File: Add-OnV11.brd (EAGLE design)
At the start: 33.2 x 17.6 mm, 9 parts

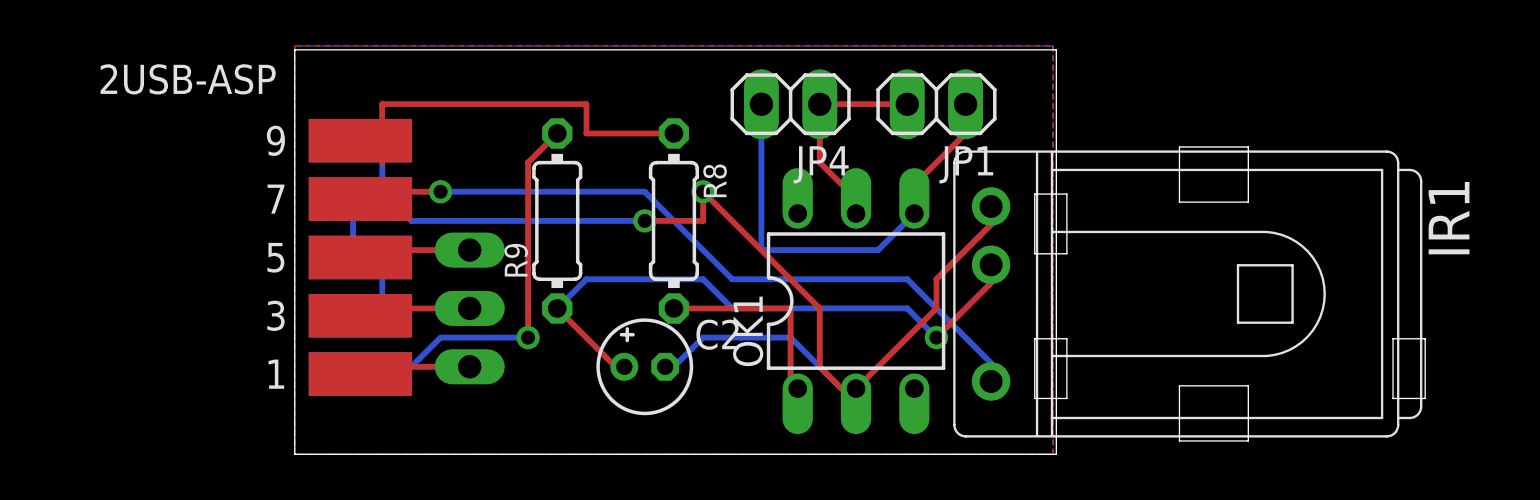
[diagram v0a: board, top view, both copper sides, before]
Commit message: Optimized
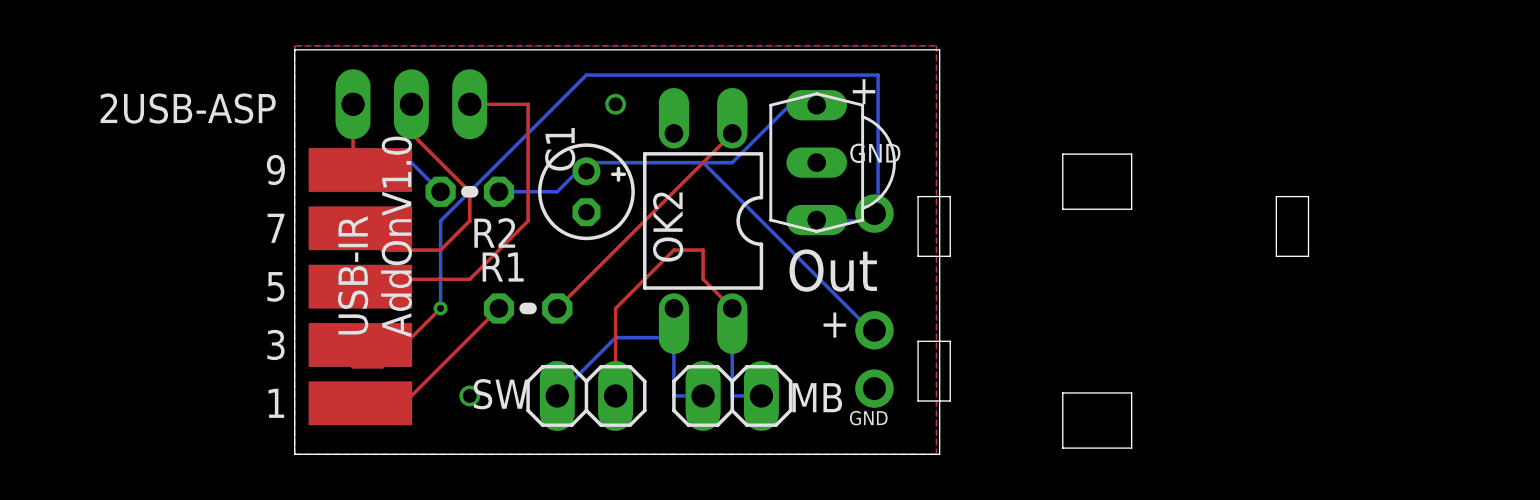
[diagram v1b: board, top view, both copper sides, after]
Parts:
- removed C2: 4,7uF, rcl:E1,8-4
- removed JP1, JP4: (no value), pinhead:1X02
- removed OK1: CNY17, optocoupler:DIL06
- removed R8: 100, rcl:0204/7
- removed R9: 560, rcl:0204/7
- added C1: 4,7uF, rcl:E1,8-4
- added MB, SW: (no value), pinhead:1X02
- added OK2: PC817, optocoupler:DIL04
- added R1: 100, rcl:0204V
- added R2: 560, rcl:0204V
- added U$1: TSOP1838, tsop-1:TSOP18XX
- moved FREI 9.25 mm to (5.08, 15.2), turned to 180 degrees
- moved IR1 5.09 mm to (25.2, 6.67), flipped to the bottom, turned to 0 degrees
- moved 2USB-ASP 1.27 mm to (2.86, 7.30)
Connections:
- removed net N$5: 2USB-ASP.P$2, R9.2
- removed net N$6: 2USB-ASP.P$5, FREI.1
- removed net N$7: 2USB-ASP.P$3, FREI.2
- removed net N$8: 2USB-ASP.P$1, FREI.3
- new net MOSI: 2USB-ASP.P$9, FREI.1
- new net NC: 2USB-ASP.P$7, FREI.2
- new net RST: 2USB-ASP.P$5, FREI.3
- new net VCC: 2USB-ASP.P$10, R2.2
- net GND: now also 2USB-ASP.P$2, C1.-, OK2.2, U$1.GND; no longer 2USB-ASP.P$10, C2.-, OK1.2
- net MISO: now also 2USB-ASP.P$1, R1.1; no longer 2USB-ASP.P$9, R8.1
- net N$1: now also C1.+, R2.1, U$1.VCC; no longer C2.+, R9.1
- net N$2: now also OK2.1, R1.2; no longer OK1.1, R8.2
- net N$3: now also MB.2, OK2.4, SW.1; no longer JP1.2, JP4.1, OK1.5
- net N$4: now also MB.1, OK2.3, SW.2; no longer JP1.1, JP4.2, OK1.4
- net SCK: now also 2USB-ASP.P$3, U$1.OUT; no longer 2USB-ASP.P$7
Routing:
- net GND: track 65.4 -> 0.00 mm
- net N$5: track 17.3 -> 0.00 mm, vias 1 -> 0
- net RST: track 0.00 -> 16.0 mm
- net NC: track 0.00 -> 12.7 mm
- net SCK: track 31.5 -> 41.5 mm
- net MISO: track 17.5 -> 7.66 mm
- net N$4: track 19.5 -> 11.2 mm
- net N$3: track 9.15 -> 16.8 mm
- net N$8: track 4.81 -> 0.00 mm
- net N$7: track 4.81 -> 0.00 mm
- net N$6: track 4.81 -> 0.00 mm
- net VCC: track 0.00 -> 4.07 mm
- net MOSI: track 0.00 -> 2.99 mm
- net N$2: track 9.34 -> 10.8 mm
- net N$1: track 26.3 -> 26.9 mm, vias 1 -> 0
- added copper zone on layer 1, net GND
- added copper zone on layer 16, net GND
- removed copper zone on layer 16, net N$10
- removed copper zone on layer 1, net N$9
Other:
- board size 33.2 x 17.6 mm -> 28.1 x 17.6 mm
- board text added: "+"
- board text added: "GND"
- board text added: "Out"
- board text added: "USB-IR AddOnV1.0"
